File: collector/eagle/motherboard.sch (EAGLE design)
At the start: 9 parts

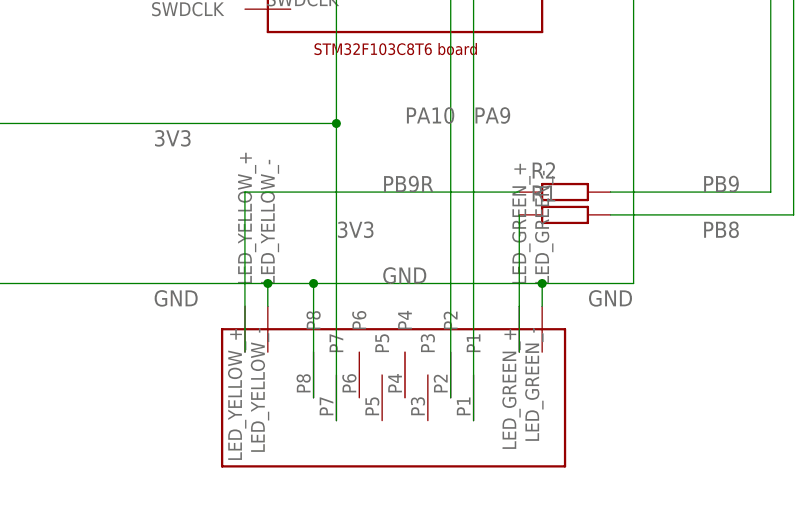
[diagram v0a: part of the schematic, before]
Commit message: Updated scheme of collector motherboard
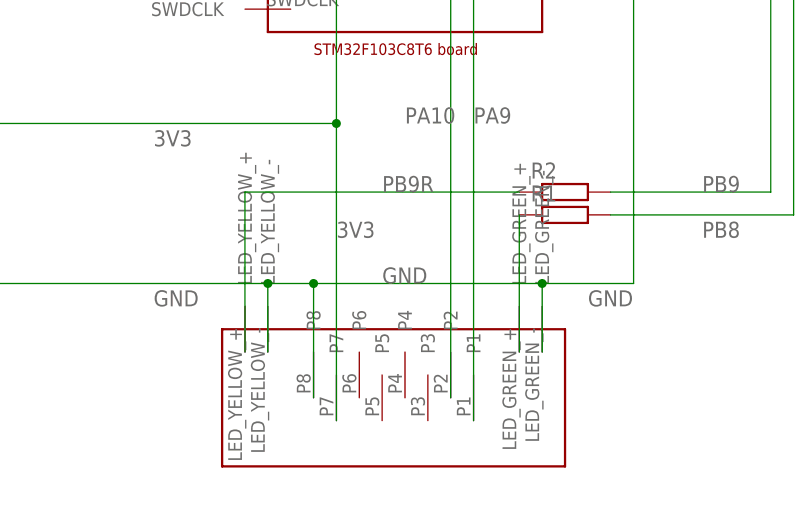
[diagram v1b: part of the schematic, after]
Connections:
- net GND: now also U$3.LED_GREEN_-, U$3.LED_YELLOW_-
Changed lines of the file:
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@@
 <part name="U$1" library="ut-boards" deviceset="HANRUN_HR911105A_15/10" device=""/>
 <part name="U$2" library="ut-boards" deviceset="STM32F103C8T6_BOARD_BLACK" device=""/>
-<part name="U$3" library="ut-connectors" deviceset="RJHSE-5481_(RJ45)" device=""/>
 <part name="R1" library="resistor" deviceset="R-EU_" device="R1206"/>
 <part name="R2" library="resistor" deviceset="R-EU_" device="R1206"/>
@@
 <part name="R4" library="resistor" deviceset="R-EU_" device="R1206"/>
 <part name="R5" library="resistor" deviceset="R-EU_" device="R1206"/>
+<part name="U$3" library="ut-connectors" deviceset="RJHSE-5481_(RJ45)" device=""/>
 </parts>
 <sheets>
@@
 <instance part="U$1" gate="G$1" x="40.64" y="60.96" rot="R270"/>
 <instance part="U$2" gate="G$1" x="104.14" y="43.18"/>
-<instance part="U$3" gate="G$1" x="101.6" y="-35.56"/>
 <instance part="R1" gate="G$1" x="121.92" y="-12.7"/>
 <instance part="R2" gate="G$1" x="121.92" y="-10.16"/>
@@
 <instance part="R4" gate="G$1" x="76.2" y="33.02"/>
 <instance part="R5" gate="G$1" x="76.2" y="38.1"/>
+<instance part="U$3" gate="G$1" x="101.6" y="-35.56"/>
 </instances>
 <busses>
@@
 <wire x1="119.38" y1="-20.32" x2="93.98" y2="-20.32" width="0.1524" layer="91"/>
 <wire x1="93.98" y1="-20.32" x2="88.9" y2="-20.32" width="0.1524" layer="91"/>
-<wire x1="88.9" y1="-20.32" x2="88.9" y2="-22.86" width="0.1524" layer="91"/>
-<wire x1="119.38" y1="-20.32" x2="119.38" y2="-22.86" width="0.1524" layer="91"/>
 <junction x="88.9" y="-20.32"/>
 <wire x1="129.54" y1="-20.32" x2="119.38" y2="-20.32" width="0.1524" layer="91"/>
@@
 <wire x1="93.98" y1="-33.02" x2="93.98" y2="-20.32" width="0.1524" layer="91"/>
 <junction x="93.98" y="-20.32"/>
-<pinref part="U$3" gate="G$1" pin="P8"/>
 <wire x1="88.9" y1="-20.32" x2="35.56" y2="-20.32" width="0.1524" layer="91"/>
 <wire x1="35.56" y1="-20.32" x2="35.56" y2="45.72" width="0.1524" layer="91"/>
@@
 <label x="124.46" y="-22.86" size="1.778" layer="95"/>
 <label x="101.6" y="-20.32" size="1.778" layer="95"/>
+<pinref part="U$3" gate="G$1" pin="P8"/>
+<pinref part="U$3" gate="G$1" pin="LED_YELLOW_-"/>
+<wire x1="88.9" y1="-20.32" x2="88.9" y2="-27.94" width="0.1524" layer="91"/>
+<pinref part="U$3" gate="G$1" pin="LED_GREEN_-"/>
+<wire x1="119.38" y1="-20.32" x2="119.38" y2="-27.94" width="0.1524" layer="91"/>
 </segment>
 </net>
@@
 <wire x1="116.84" y1="27.94" x2="96.52" y2="27.94" width="0.1524" layer="91"/>
 <wire x1="96.52" y1="27.94" x2="96.52" y2="-2.54" width="0.1524" layer="91"/>
-<pinref part="U$3" gate="G$1" pin="P7"/>
 <wire x1="96.52" y1="-2.54" x2="96.52" y2="-35.56" width="0.1524" layer="91"/>
 <wire x1="96.52" y1="-2.54" x2="38.1" y2="-2.54" width="0.1524" layer="91"/>
@@
 <label x="76.2" y="-5.08" size="1.778" layer="95"/>
 <label x="96.52" y="-15.24" size="1.778" layer="95"/>
+<pinref part="U$3" gate="G$1" pin="P7"/>
 </segment>
 </net>
@@
 <net name="N$9" class="0">
 <segment>
-<wire x1="116.84" y1="-12.7" x2="116.84" y2="-22.86" width="0.1524" layer="91"/>
+<wire x1="116.84" y1="-12.7" x2="116.84" y2="-27.94" width="0.1524" layer="91"/>
+<pinref part="R1" gate="G$1" pin="1"/>
 <pinref part="U$3" gate="G$1" pin="LED_GREEN_+"/>
-<pinref part="R1" gate="G$1" pin="1"/>
-<wire x1="116.84" y1="-27.94" x2="116.84" y2="-22.86" width="0.1524" layer="91"/>
 </segment>
 </net>
@@
 <segment>
 <wire x1="86.36" y1="-10.16" x2="86.36" y2="-27.94" width="0.1524" layer="91"/>
-<pinref part="U$3" gate="G$1" pin="LED_YELLOW_+"/>
 <pinref part="R2" gate="G$1" pin="1"/>
 <wire x1="116.84" y1="-10.16" x2="86.36" y2="-10.16" width="0.1524" layer="91"/>
 <label x="101.6" y="-10.16" size="1.778" layer="95"/>
+<pinref part="U$3" gate="G$1" pin="LED_YELLOW_+"/>
 </segment>
 </net>
@@
 <junction x="91.44" y="58.42"/>
 <wire x1="111.76" y1="58.42" x2="111.76" y2="-35.56" width="0.1524" layer="91"/>
+<label x="111.76" y="-2.54" size="1.778" layer="95"/>
 <pinref part="U$3" gate="G$1" pin="P1"/>
-<label x="111.76" y="-2.54" size="1.778" layer="95"/>
 </segment>
 </net>
@@
 <junction x="91.44" y="55.88"/>
 <wire x1="109.22" y1="55.88" x2="109.22" y2="-33.02" width="0.1524" layer="91"/>
+<label x="104.14" y="-2.54" size="1.778" layer="95"/>
 <pinref part="U$3" gate="G$1" pin="P2"/>
-<label x="104.14" y="-2.54" size="1.778" layer="95"/>
 </segment>
 </net>

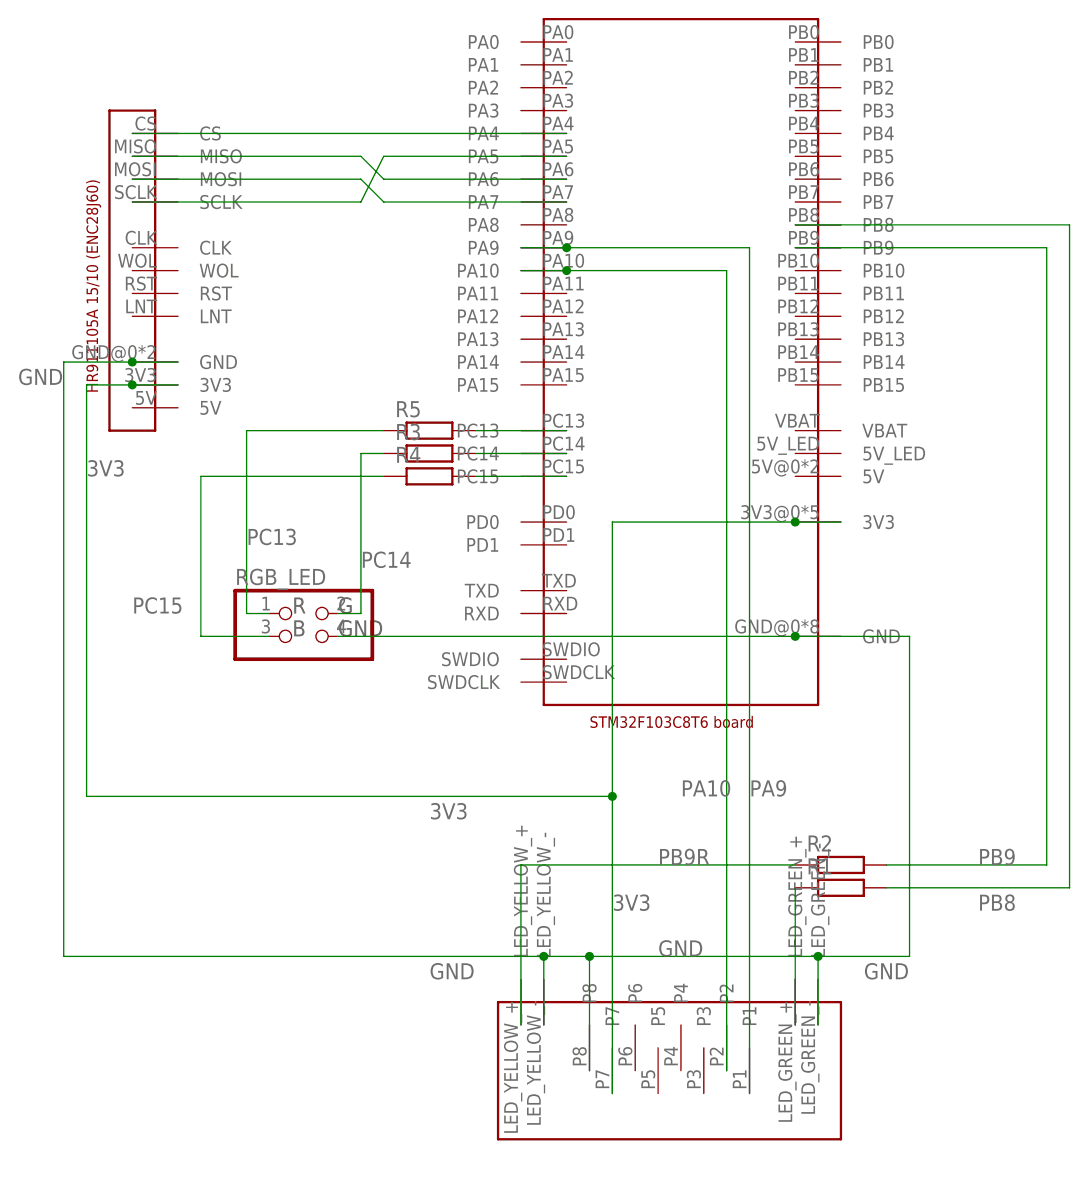
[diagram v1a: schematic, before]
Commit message: Tiny fixes on colletor's motherboard
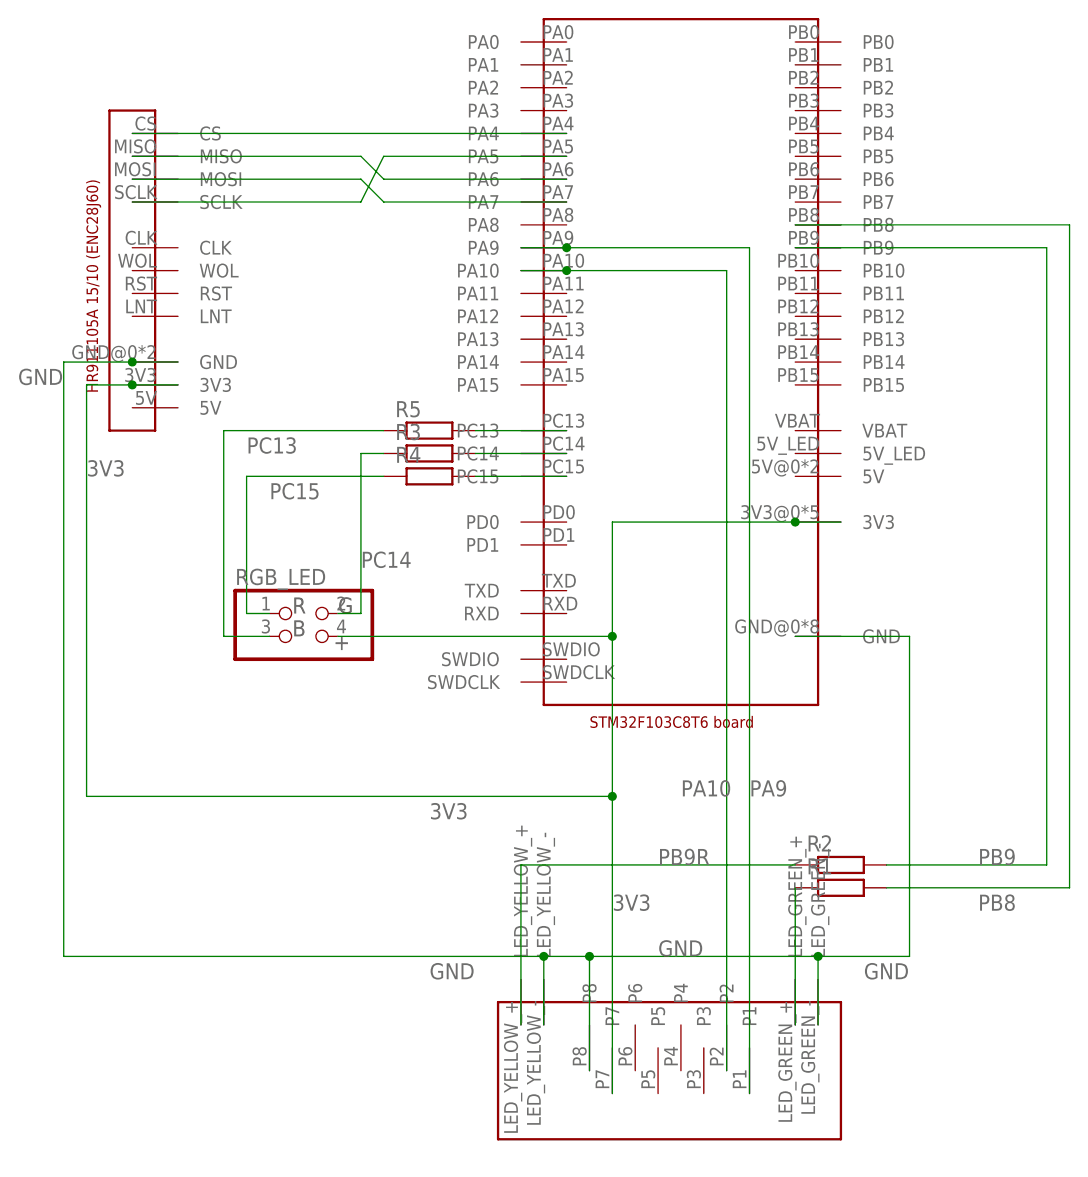
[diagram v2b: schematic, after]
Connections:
- net 3V3: now also RGB_LED.4
- net GND: no longer RGB_LED.4
- net PC13: now also RGB_LED.3; no longer RGB_LED.1
- net PC15: now also RGB_LED.1; no longer RGB_LED.3
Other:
- note added: "+"
- note removed: "GND"
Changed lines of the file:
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@@
 <text x="66.04" y="17.78" size="1.778" layer="97">G</text>
 <text x="60.96" y="15.24" size="1.778" layer="97">B</text>
-<text x="66.04" y="15.24" size="1.778" layer="97">GND</text>
+<text x="65.532" y="13.716" size="1.778" layer="97">+</text>
 </plain>
 <instances>
@@
 <wire x1="129.54" y1="-20.32" x2="119.38" y2="-20.32" width="0.1524" layer="91"/>
 <junction x="119.38" y="-20.32"/>
-<pinref part="RGB_LED" gate="A" pin="4"/>
-<wire x1="66.04" y1="15.24" x2="116.84" y2="15.24" width="0.1524" layer="91"/>
-<junction x="116.84" y="15.24"/>
 <wire x1="93.98" y1="-33.02" x2="93.98" y2="-20.32" width="0.1524" layer="91"/>
 <junction x="93.98" y="-20.32"/>
@@
 <junction x="116.84" y="27.94"/>
 <wire x1="116.84" y1="27.94" x2="96.52" y2="27.94" width="0.1524" layer="91"/>
-<wire x1="96.52" y1="27.94" x2="96.52" y2="-2.54" width="0.1524" layer="91"/>
+<wire x1="96.52" y1="27.94" x2="96.52" y2="15.24" width="0.1524" layer="91"/>
+<wire x1="96.52" y1="15.24" x2="96.52" y2="-2.54" width="0.1524" layer="91"/>
 <wire x1="96.52" y1="-2.54" x2="96.52" y2="-35.56" width="0.1524" layer="91"/>
 <wire x1="96.52" y1="-2.54" x2="38.1" y2="-2.54" width="0.1524" layer="91"/>
@@
 <label x="96.52" y="-15.24" size="1.778" layer="95"/>
 <pinref part="U$3" gate="G$1" pin="P7"/>
+<pinref part="RGB_LED" gate="A" pin="4"/>
+<wire x1="96.52" y1="15.24" x2="66.04" y2="15.24" width="0.1524" layer="91"/>
+<junction x="96.52" y="15.24"/>
 </segment>
 </net>
@@
 <net name="PC13" class="0">
 <segment>
-<pinref part="RGB_LED" gate="A" pin="1"/>
-<wire x1="55.88" y1="38.1" x2="55.88" y2="17.78" width="0.1524" layer="91"/>
-<wire x1="55.88" y1="17.78" x2="58.42" y2="17.78" width="0.1524" layer="91"/>
 <pinref part="R5" gate="G$1" pin="1"/>
-<wire x1="71.12" y1="38.1" x2="55.88" y2="38.1" width="0.1524" layer="91"/>
-<label x="55.88" y="25.4" size="1.778" layer="95"/>
+<wire x1="71.12" y1="38.1" x2="53.34" y2="38.1" width="0.1524" layer="91"/>
+<wire x1="53.34" y1="38.1" x2="53.34" y2="15.24" width="0.1524" layer="91"/>
+<pinref part="RGB_LED" gate="A" pin="3"/>
+<wire x1="53.34" y1="15.24" x2="58.42" y2="15.24" width="0.1524" layer="91"/>
+<label x="55.88" y="35.56" size="1.778" layer="95"/>
 </segment>
 </net>
@@
 </segment>
 </net>
-<net name="PC15" class="0">
-<segment>
-<pinref part="RGB_LED" gate="A" pin="3"/>
-<wire x1="50.8" y1="33.02" x2="50.8" y2="15.24" width="0.1524" layer="91"/>
-<wire x1="50.8" y1="15.24" x2="58.42" y2="15.24" width="0.1524" layer="91"/>
-<pinref part="R4" gate="G$1" pin="1"/>
-<wire x1="71.12" y1="33.02" x2="50.8" y2="33.02" width="0.1524" layer="91"/>
-<label x="43.18" y="17.78" size="1.778" layer="95"/>
-</segment>
-</net>
 <net name="N$16" class="0">
 <segment>
@@
 </segment>
 </net>
+<net name="PC15" class="0">
+<segment>
+<pinref part="R4" gate="G$1" pin="1"/>
+<wire x1="71.12" y1="33.02" x2="55.88" y2="33.02" width="0.1524" layer="91"/>
+<wire x1="55.88" y1="33.02" x2="55.88" y2="17.78" width="0.1524" layer="91"/>
+<pinref part="RGB_LED" gate="A" pin="1"/>
+<wire x1="55.88" y1="17.78" x2="58.42" y2="17.78" width="0.1524" layer="91"/>
+<label x="58.42" y="30.48" size="1.778" layer="95"/>
+</segment>
+</net>
